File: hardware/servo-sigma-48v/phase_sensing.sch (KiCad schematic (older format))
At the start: 31 parts, among them U10 OPA4374, U9 OPA4374

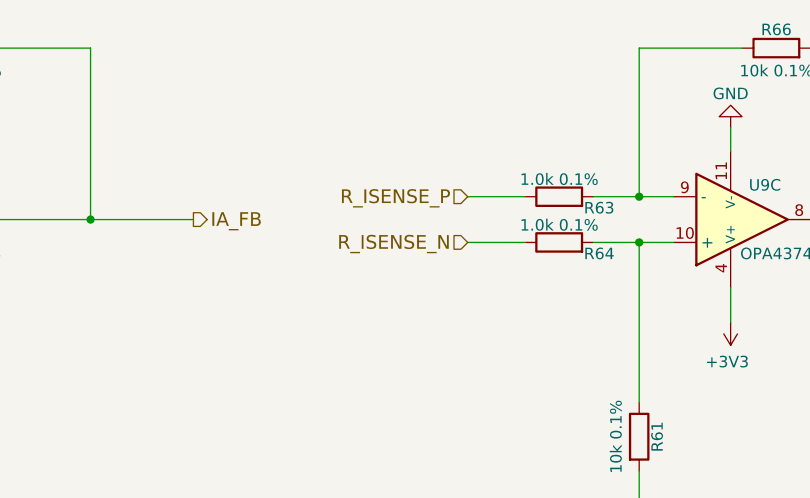
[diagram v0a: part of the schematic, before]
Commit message: Work on verson 2.0
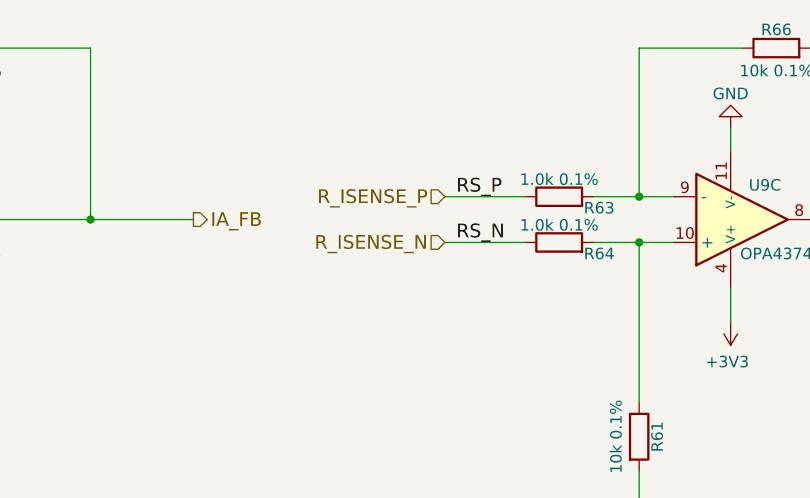
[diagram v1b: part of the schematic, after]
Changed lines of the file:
@@
 C_ISENSE_N
 Wire Wire Line
-	13000 2250 13250 2250
-Wire Wire Line
-	13000 2450 13250 2450
+	12900 2250 13250 2250
+Wire Wire Line
+	12900 2450 13250 2450
 Text HLabel 4850 2350 2    60   Output ~ 0
 IC_FB
@@
 	-1   0    0    1
 $EndComp
-Text HLabel 13000 2250 0    60   Input ~ 0
+Text HLabel 12900 2250 0    60   Input ~ 0
 R_ISENSE_P
-Text HLabel 13000 2450 0    60   Input ~ 0
+Text HLabel 12900 2450 0    60   Input ~ 0
 R_ISENSE_N
 Wire Wire Line
@@
 Wire Wire Line
 	8750 6550 12300 6550
+Text Label 12950 2250 0    60   ~ 0
+RS_P
+Text Label 12950 2450 0    60   ~ 0
+RS_N
 $EndSCHEMATC

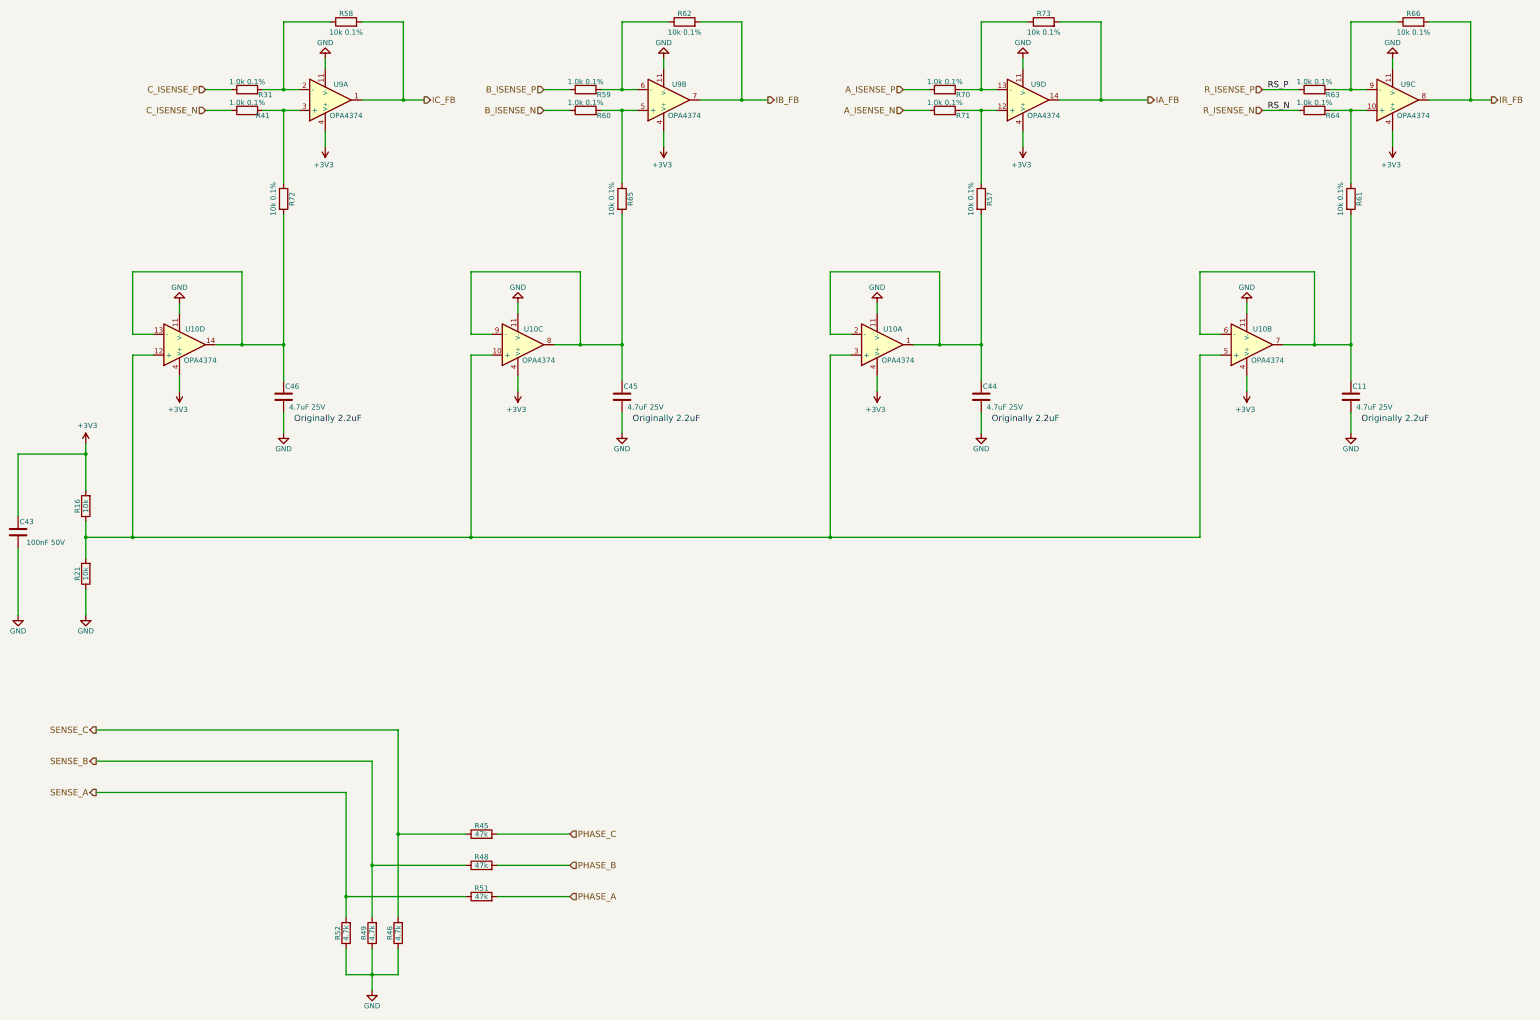
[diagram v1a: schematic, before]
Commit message: completed routing
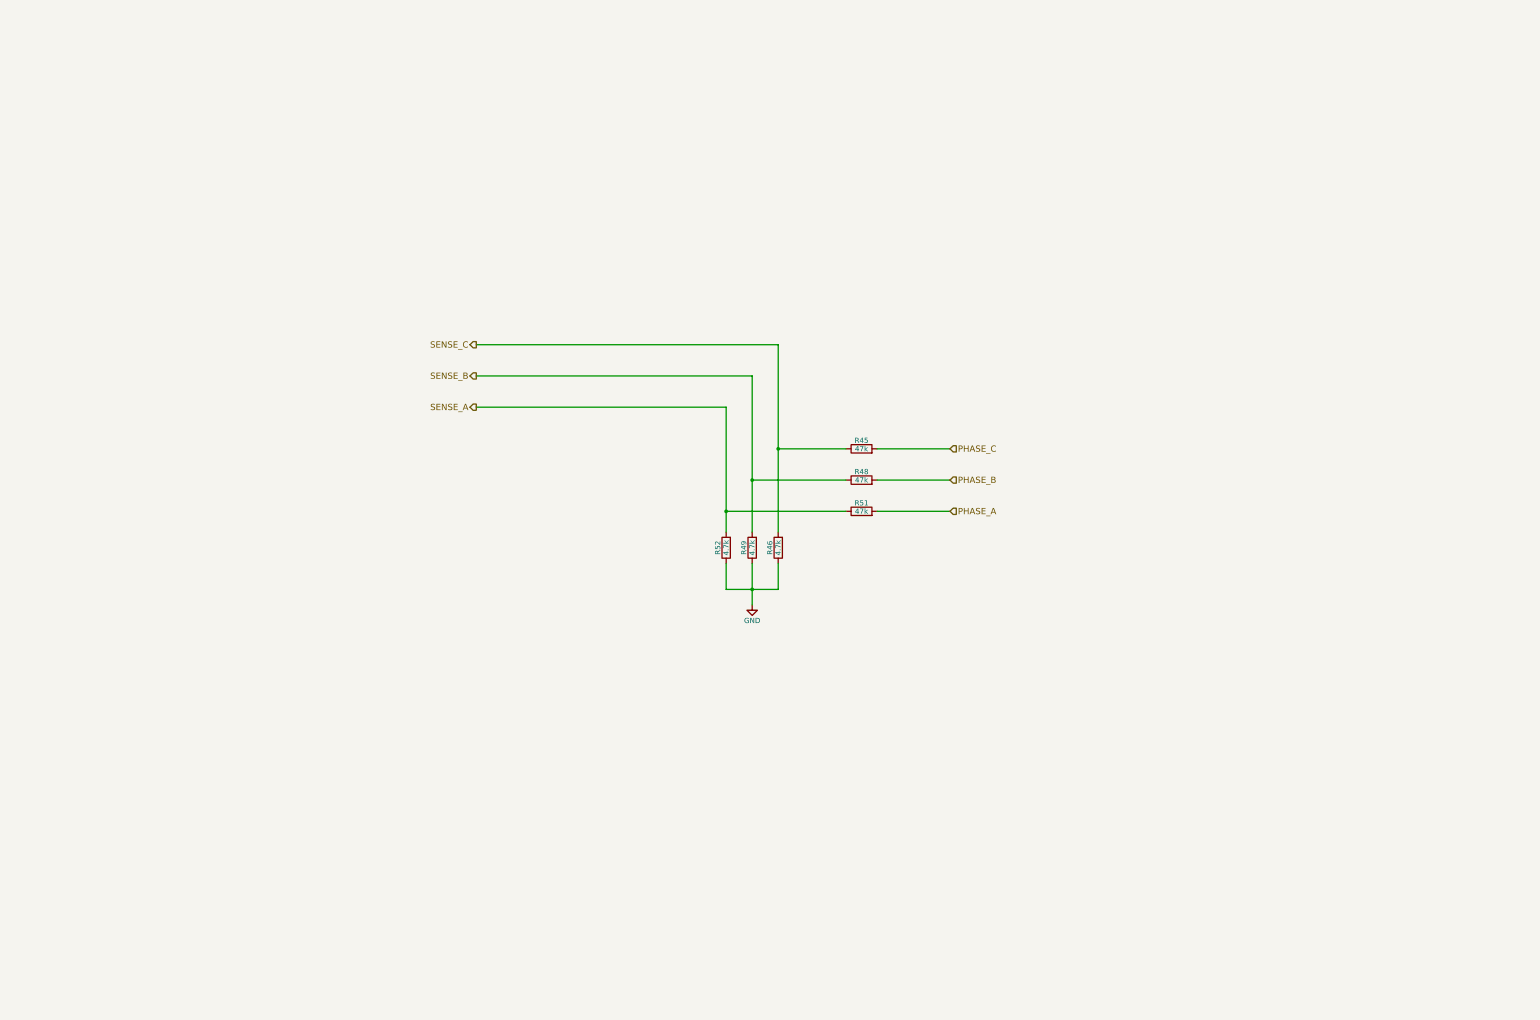
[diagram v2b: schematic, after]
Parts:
- removed C11, C44, C45, C46: 4.7uF 25V, Capacitor_SMD:C_0805_2012Metric, symbol servo-sigma-48v-rescue:C-device
- removed C43: 100nF 50V, Capacitor_SMD:C_0603_1608Metric, symbol servo-sigma-48v-rescue:C-device
- removed R16, R21: 10k, Resistor_SMD:R_0603_1608Metric, symbol servo-sigma-48v-rescue:R-device
- removed R31, R41, R59, R60, R63, R64, R70, R71: 1.0k 0.1%, Resistor_SMD:R_0603_1608Metric, symbol servo-sigma-48v-rescue:R-device
- removed R57, R58, R61, R62, R65, R66, R72, R73: 10k 0.1%, Resistor_SMD:R_0603_1608Metric, symbol servo-sigma-48v-rescue:R-device
- removed U10, U9: OPA4374, Package_SO:SOIC-14_3.9x8.7mm_P1.27mm, symbol sigmadrone:OPA4374
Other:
- note removed: "Originally 2.2uF"
- moved on the sheet: R45, R46, R48, R49, R51, R52
